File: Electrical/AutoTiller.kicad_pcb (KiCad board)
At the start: 4 copper layers, 100 x 64 mm, 69 parts, among them J1 3220-14-0300-00, J2 USB_C_Receptacle_USB2.0, J3 T4145415031-001, SW1 DS04-254-2L-01BK, SW2 TS04-66-65-BK-160-SMT, SW3 TS04-66-65-BK-160-SMT, SW4 TS04-66-65-BK-160-SMT, SW5 TS04-66-65-BK-160-SMT, SW6 TS04-66-65-BK-160-SMT, SW7 TS04-66-65-BK-160-SMT, U1 STM32F103T6Ux, U2 TUSB320LAI, U3 IIS2MDCTR, U4 MAX22201, U5 BHTGA-A-DW, U6 VO615A-4, U7 TLV76733DRVx, Y1 16 MHz

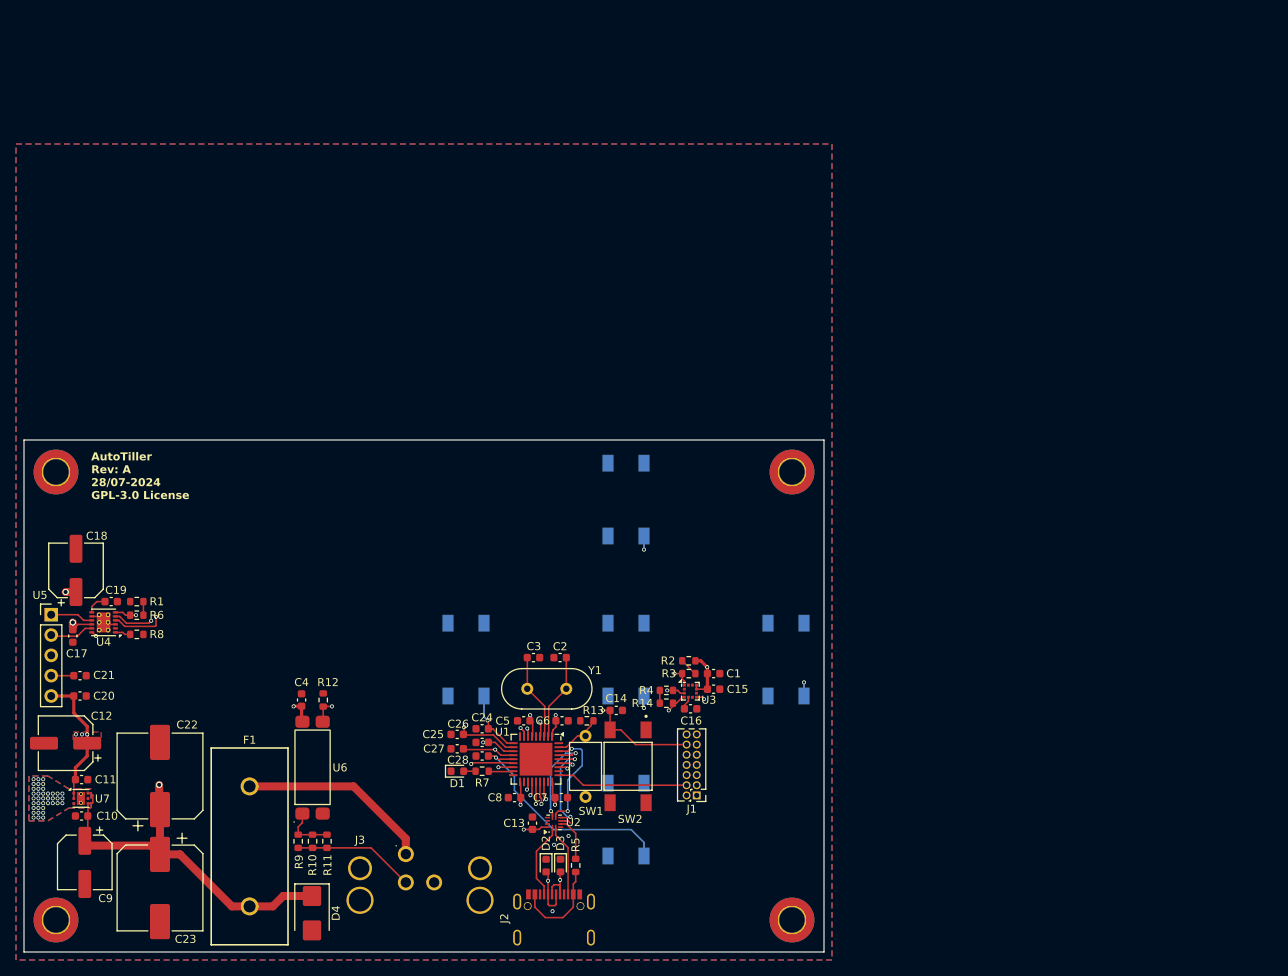
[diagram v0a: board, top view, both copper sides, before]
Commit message: Finalizing the layout
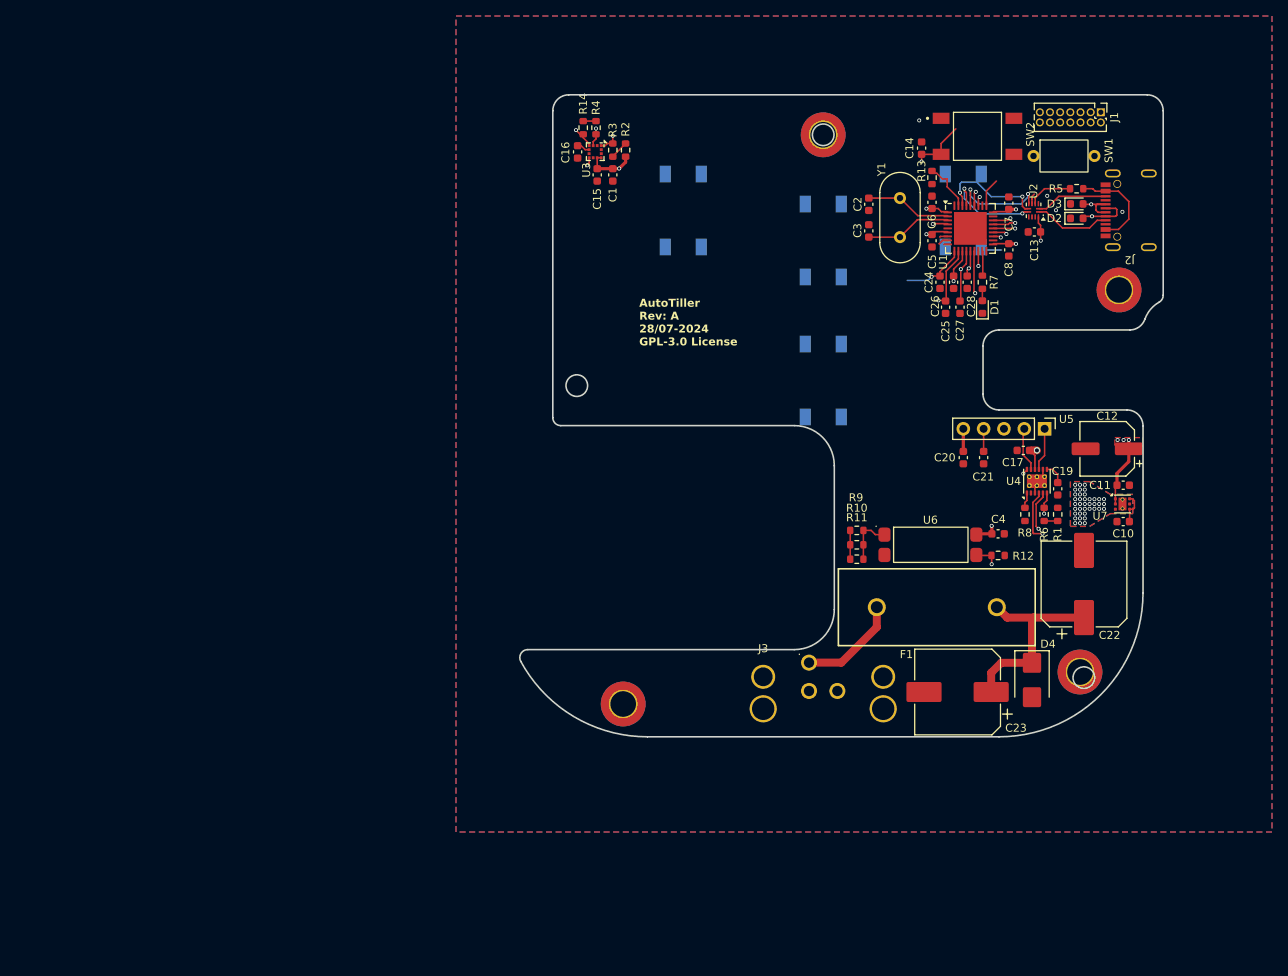
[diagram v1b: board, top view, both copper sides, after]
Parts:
- removed C18, C9: 47uF, Capacitor_SMD:CP_Elec_6.3x7.7
- removed SW3: TS04-66-65-BK-160-SMT, AutoTiller:TS04-66-65-BK-160-SMT
- SW4, SW5, SW6, SW7: value TS04-66-65-BK-160-SMT -> TS04-66-95-BK-260-SMT
- moved C10 135.3 mm to (248.4, 96.2)
- moved C11 135.3 mm to (248.4, 91.7)
- moved C12 135.3 mm to (246.4, 87.1)
- moved U7 135.3 mm to (248.3, 94.0)
- moved U5 126.3 mm to (238.6, 84.6), turned to -90 degrees
- moved C17 121.1 mm to (235.9, 87.3), turned to 180 degrees
- moved C19 119.2 mm to (240.2, 92.1), turned to -90 degrees
- moved U4 118.0 mm to (237.6, 91.2), turned to 90 degrees
- moved C22 118.0 mm to (243.5, 104.0)
- moved J2 117.5 mm to (251.6, 57.2), turned to 90 degrees
- moved C21 116.2 mm to (231.0, 88.2), turned to -90 degrees
- moved R1 115.6 mm to (240.2, 95.3), turned to -90 degrees
- moved C20 114.4 mm to (228.4, 88.2), turned to -90 degrees
- moved R6 114.1 mm to (238.5, 95.3), turned to 90 degrees
- moved R8 112.0 mm to (236.1, 95.3), turned to 90 degrees
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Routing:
- net /Motor Driver/IN1: track 59.9 -> 7.82 mm, vias 2 -> 1
- net /Motor Driver/IN2: track 57.9 -> 6.48 mm, vias 2 -> 1
- net /Processor/ACTUATOR_POT: track 65.2 -> 15.9 mm
- net VDD: track 81.8 -> 33.1 mm, vias 3 -> 1
- net /Motor Driver/FAULT: track 68.3 -> 22.2 mm
- net /Motor Driver/ISEN: track 57.9 -> 17.5 mm
- net Net-(U1-PA7): track 28.9 -> 3.28 mm
- net Net-(U1-PA6): track 55.0 -> 30.3 mm, vias 2 -> 1
- net UART_RX: track 57.1 -> 34.5 mm
- net Net-(U1-PA4): track 52.1 -> 33.4 mm, vias 2 -> 1
- net /Processor/SWCLK: track 21.1 -> 7.39 mm
- net /Processor/SWDIO: track 16.5 -> 3.61 mm
- net /E-Compass/I2C_SCL: track 34.2 -> 22.3 mm
- net Net-(J3-Pin_2): track 15.2 -> 3.60 mm
- net /E-Compass/INT/DRDY: track 22.7 -> 11.2 mm
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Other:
- board size 100 x 64 mm -> 80.4 x 80.2 mm
